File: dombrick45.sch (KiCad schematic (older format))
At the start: 119 parts, among them J1 AVR-ISP-6, SW1 SW_Push, U1 ATmega32U4-AU, U2 PRTR5V0U2X, Y1 16MHz

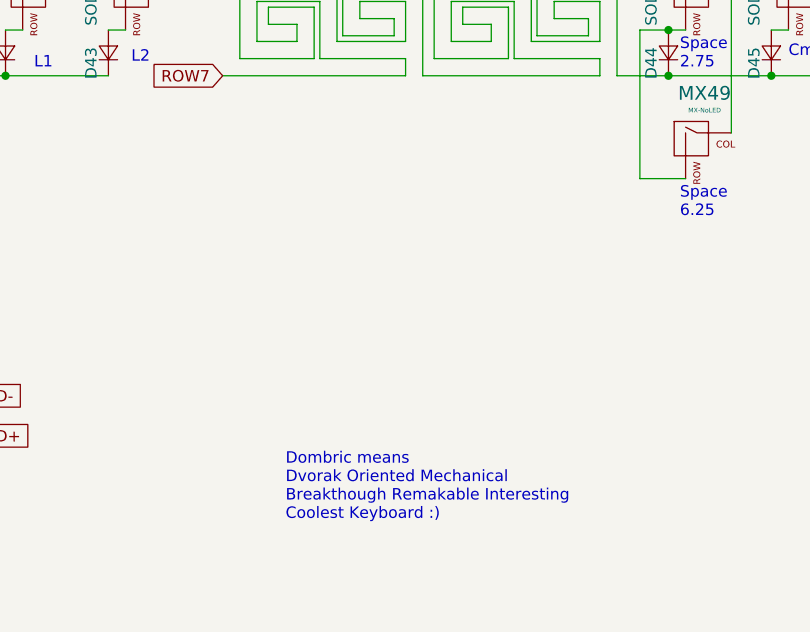
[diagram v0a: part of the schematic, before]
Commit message: 2019-10-22 hobo OK
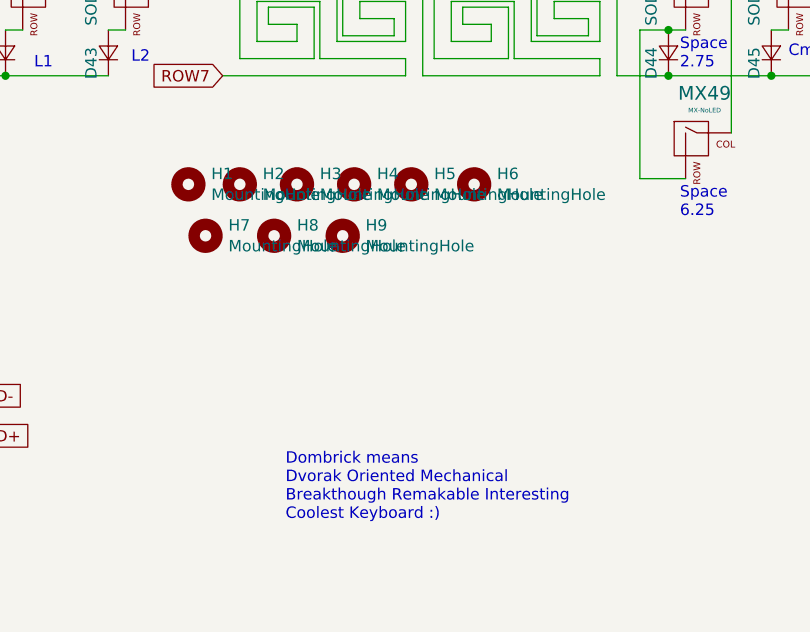
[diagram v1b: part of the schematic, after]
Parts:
- added H1, H2, H3, H4, H5, H6, H7, H8, H9: MountingHole, MountingHole:MountingHole_2.2mm_M2, symbol Mechanical:MountingHole
- MX44: footprint MX_Only:MXOnly-2.75U-Hotswap-ReversedStabilizers -> MX_Only:MXOnly-2.75U-Hotswap
- MX49: footprint MX_Only:MXOnly-6.25U-Hotswap -> MX_Only:MXOnly-6.25U-Hotswap-ReversedStabilizers
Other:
- note added: "Dombrick means \nDvorak Oriented Mechanical\nBreakthough Remakable Interesting\nCoolest Keyboard :)"
- note removed: "Dombric means \nDvorak Oriented Mechanical\nBreakthough Remakable Interesting\nCoolest Keyboard :)"
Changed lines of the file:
@@
 COL0
 Text Notes 7025 6900 0    50   ~ 0
-Dombric means \nDvorak Oriented Mechanical\nBreakthough Remakable Interesting\nCoolest Keyboard :)
+Dombrick means \nDvorak Oriented Mechanical\nBreakthough Remakable Interesting\nCoolest Keyboard :)
 Text Notes 6850 4175 0    50   ~ 0
 X
@@
 F 0 "MX44" H 8858 4823 60  0000 C CNN
 F 1 "MX-NoLED" H 8858 4749 20  0000 C CNN
-F 2 "MX_Only:MXOnly-2.75U-Hotswap-ReversedStabilizers" H 8200 4575 60  0001 C CNN
+F 2 "MX_Only:MXOnly-2.75U-Hotswap" H 8200 4575 60  0001 C CNN
 F 3 "" H 8200 4575 60  0001 C CNN
 	1    8825 4600
@@
 F 0 "MX49" H 8858 5473 60  0000 C CNN
 F 1 "MX-NoLED" H 8858 5399 20  0000 C CNN
-F 2 "MX_Only:MXOnly-6.25U-Hotswap" H 8200 5225 60  0001 C CNN
+F 2 "MX_Only:MXOnly-6.25U-Hotswap-ReversedStabilizers" H 8200 5225 60  0001 C CNN
 F 3 "" H 8200 5225 60  0001 C CNN
 	1    8825 5250
@@
 Wire Wire Line
 	2350 6300 2125 6300
+$Comp
+L Mechanical:MountingHole H1
+U 1 1 5DCE16C5
+P 6600 5425
+F 0 "H1" H 6700 5471 50  0000 L CNN
+F 1 "MountingHole" H 6700 5380 50  0000 L CNN
+F 2 "MountingHole:MountingHole_2.2mm_M2" H 6600 5425 50  0001 C CNN
+F 3 "~" H 6600 5425 50  0001 C CNN
+	1    6600 5425
+	1    0    0    -1
+$EndComp
+$Comp
+L Mechanical:MountingHole H2
+U 1 1 5DCE1A14
+P 6825 5425
+F 0 "H2" H 6925 5471 50  0000 L CNN
+F 1 "MountingHole" H 6925 5380 50  0000 L CNN
+F 2 "MountingHole:MountingHole_2.2mm_M2" H 6825 5425 50  0001 C CNN
+F 3 "~" H 6825 5425 50  0001 C CNN
+	1    6825 5425
+	1    0    0    -1
+$EndComp
+$Comp
+L Mechanical:MountingHole H3
+U 1 1 5DCE1D28
+P 7075 5425
+F 0 "H3" H 7175 5471 50  0000 L CNN
+F 1 "MountingHole" H 7175 5380 50  0000 L CNN
+F 2 "MountingHole:MountingHole_2.2mm_M2" H 7075 5425 50  0001 C CNN
+F 3 "~" H 7075 5425 50  0001 C CNN
+	1    7075 5425
+	1    0    0    -1
+$EndComp
+$Comp
+L Mechanical:MountingHole H4
+U 1 1 5DCE1FD6
+P 7325 5425
+F 0 "H4" H 7425 5471 50  0000 L CNN
+F 1 "MountingHole" H 7425 5380 50  0000 L CNN
+F 2 "MountingHole:MountingHole_2.2mm_M2" H 7325 5425 50  0001 C CNN
+F 3 "~" H 7325 5425 50  0001 C CNN
+	1    7325 5425
+	1    0    0    -1
+$EndComp
+$Comp
+L Mechanical:MountingHole H5
+U 1 1 5DCE231D
+P 7575 5425
+F 0 "H5" H 7675 5471 50  0000 L CNN
+F 1 "MountingHole" H 7675 5380 50  0000 L CNN
+F 2 "MountingHole:MountingHole_2.2mm_M2" H 7575 5425 50  0001 C CNN
+F 3 "~" H 7575 5425 50  0001 C CNN
+	1    7575 5425
+	1    0    0    -1
+$EndComp
+$Comp
+L Mechanical:MountingHole H6
+U 1 1 5DCE2598
+P 7850 5425
+F 0 "H6" H 7950 5471 50  0000 L CNN
+F 1 "MountingHole" H 7950 5380 50  0000 L CNN
+F 2 "MountingHole:MountingHole_2.2mm_M2" H 7850 5425 50  0001 C CNN
+F 3 "~" H 7850 5425 50  0001 C CNN
+	1    7850 5425
+	1    0    0    -1
+$EndComp
+$Comp
+L Mechanical:MountingHole H7
+U 1 1 5DCE2989
+P 6675 5650
+F 0 "H7" H 6775 5696 50  0000 L CNN
+F 1 "MountingHole" H 6775 5605 50  0000 L CNN
+F 2 "MountingHole:MountingHole_2.2mm_M2" H 6675 5650 50  0001 C CNN
+F 3 "~" H 6675 5650 50  0001 C CNN
+	1    6675 5650
+	1    0    0    -1
+$EndComp
+$Comp
+L Mechanical:MountingHole H8
+U 1 1 5DCE2D36
+P 6975 5650
+F 0 "H8" H 7075 5696 50  0000 L CNN
+F 1 "MountingHole" H 7075 5605 50  0000 L CNN
+F 2 "MountingHole:MountingHole_2.2mm_M2" H 6975 5650 50  0001 C CNN
+F 3 "~" H 6975 5650 50  0001 C CNN
+	1    6975 5650
+	1    0    0    -1
+$EndComp
+$Comp
+L Mechanical:MountingHole H9
+U 1 1 5DCE3149
+P 7275 5650
+F 0 "H9" H 7375 5696 50  0000 L CNN
+F 1 "MountingHole" H 7375 5605 50  0000 L CNN
+F 2 "MountingHole:MountingHole_2.2mm_M2" H 7275 5650 50  0001 C CNN
+F 3 "~" H 7275 5650 50  0001 C CNN
+	1    7275 5650
+	1    0    0    -1
+$EndComp
 $EndSCHEMATC
